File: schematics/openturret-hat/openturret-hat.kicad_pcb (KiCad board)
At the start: 2 copper layers, 8 parts, among them J1 Raspberry_Pi_2_3, J2 Conn_02x03_Odd_Even, U0 L293D, U1 L293D, U2 ATtiny24A-PU, U3 L7805

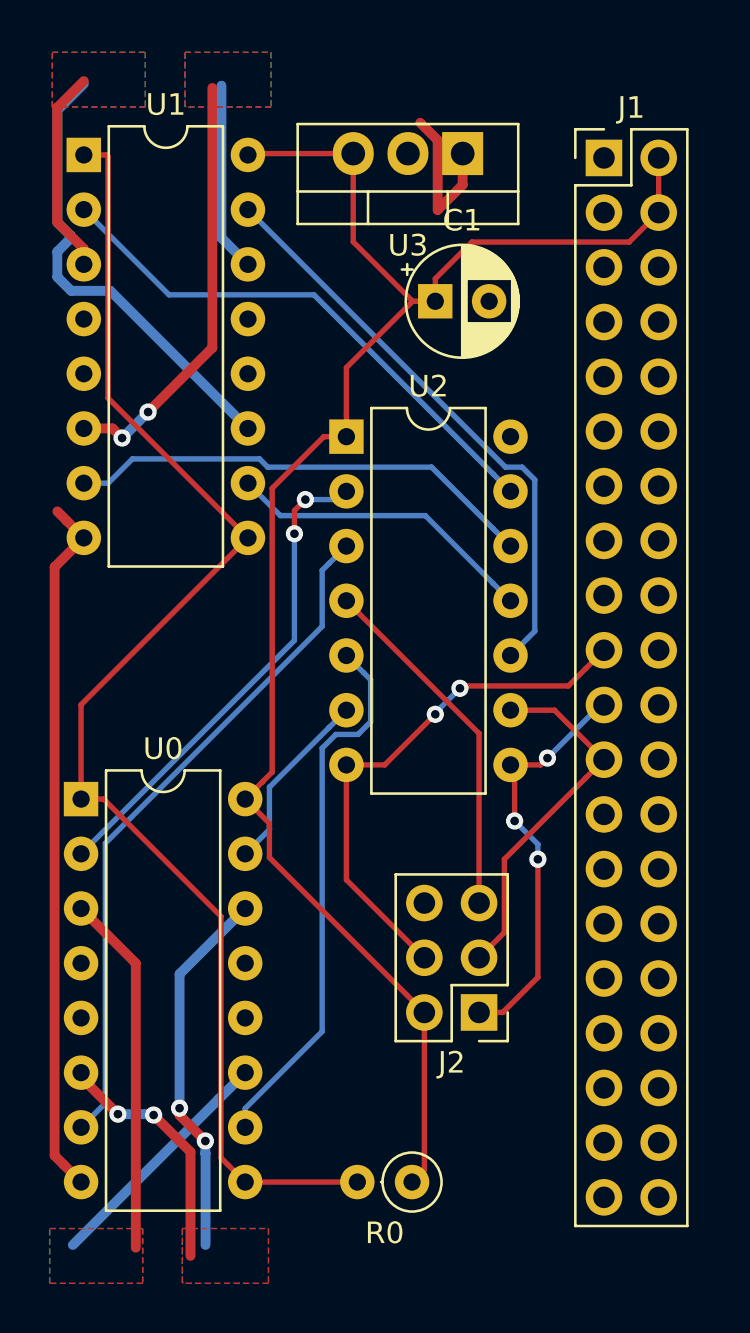
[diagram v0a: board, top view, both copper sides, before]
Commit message: openturret hat board rev 1
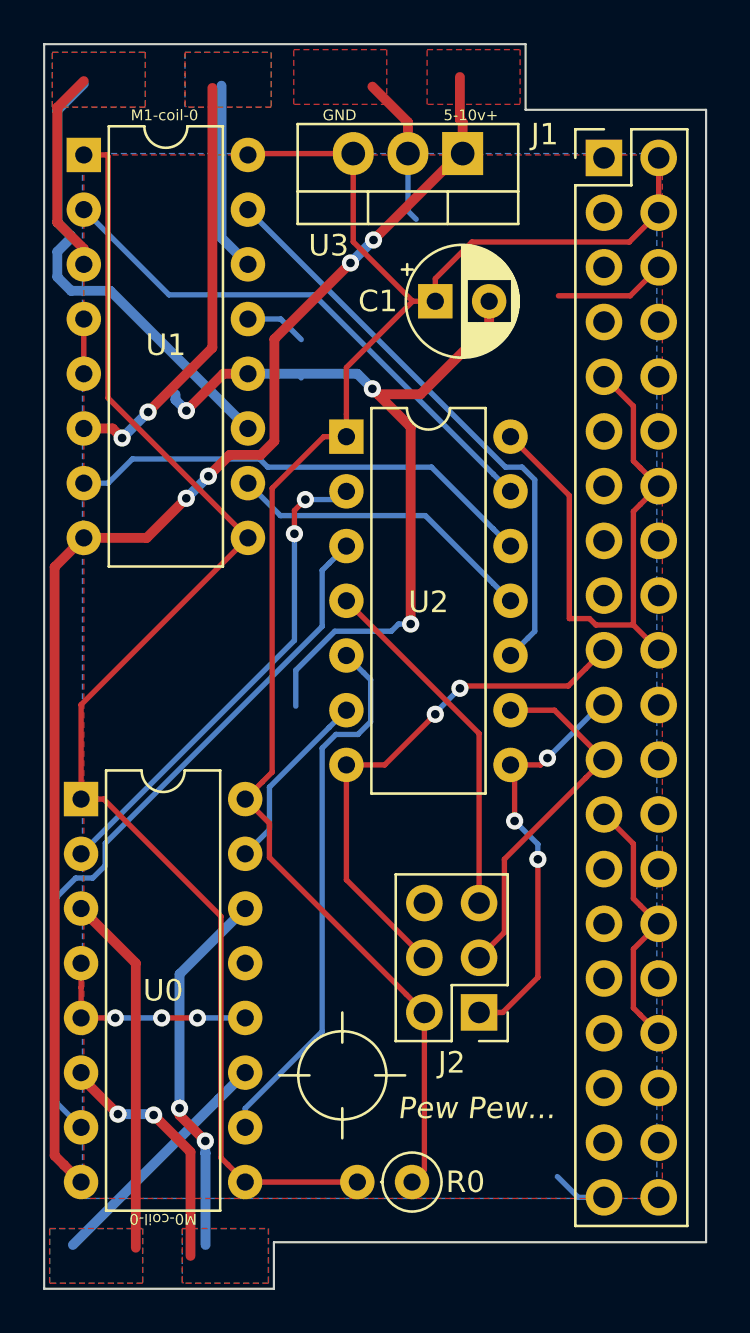
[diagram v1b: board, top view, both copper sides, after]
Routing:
- net GND: track 0.00 -> 110.6 mm, vias 0 -> 6
- net VDC: track 40.2 -> 62.3 mm, vias 0 -> 4
- net M0-coil0-1: track 32.1 -> 33.5 mm
- added copper zone on B.Cu, net GND
- added copper zone on F.Cu, net GND
- added copper zone on F.Cu, net VDC
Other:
- board outline added: 30.7 x 57.8 mm
- board text added: "5-10v+"
- board text added: "GND"
- board text added: "M0-coil-0"
- board text added: "M0-coil-1"
- board text added: "M1-coil-0"
- board text added: "M1-coil-1"
- board text added: "Pew Pew..."
